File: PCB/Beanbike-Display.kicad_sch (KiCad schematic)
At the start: 5 parts, among them J1 Conn_01x21_Socket, J2 Conn_01x21_Socket, J3 Conn_01x18_Socket, J4 Conn_01x03_Socket, J5 Conn_01x08_Socket

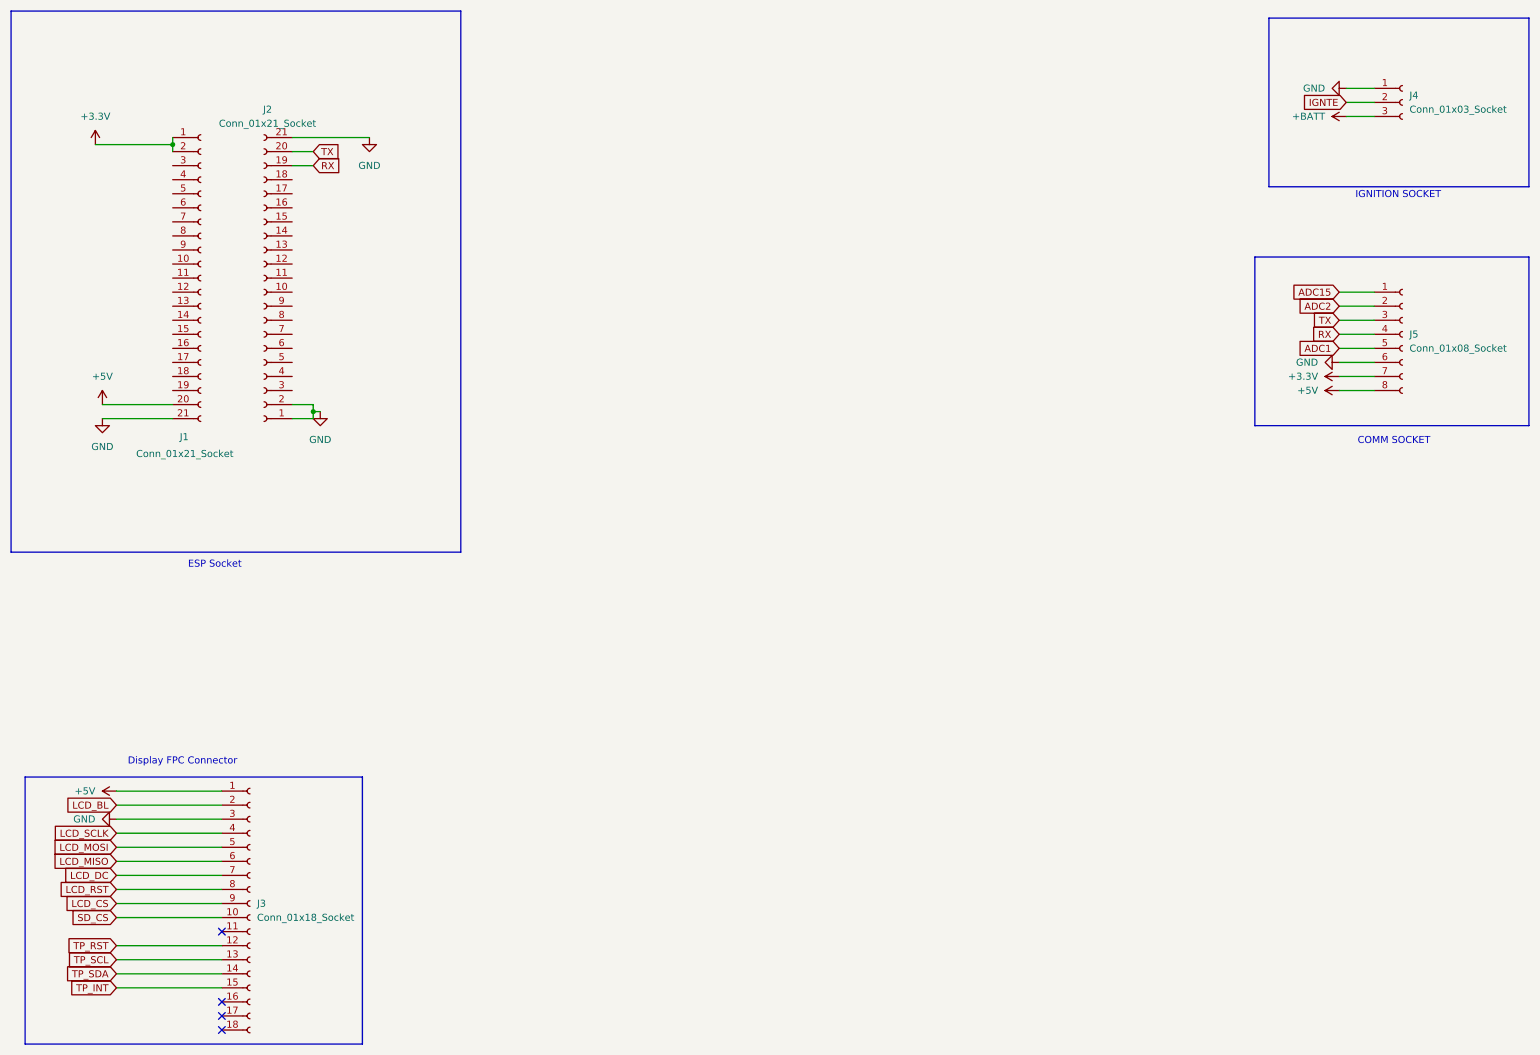
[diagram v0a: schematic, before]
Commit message: PCB v1
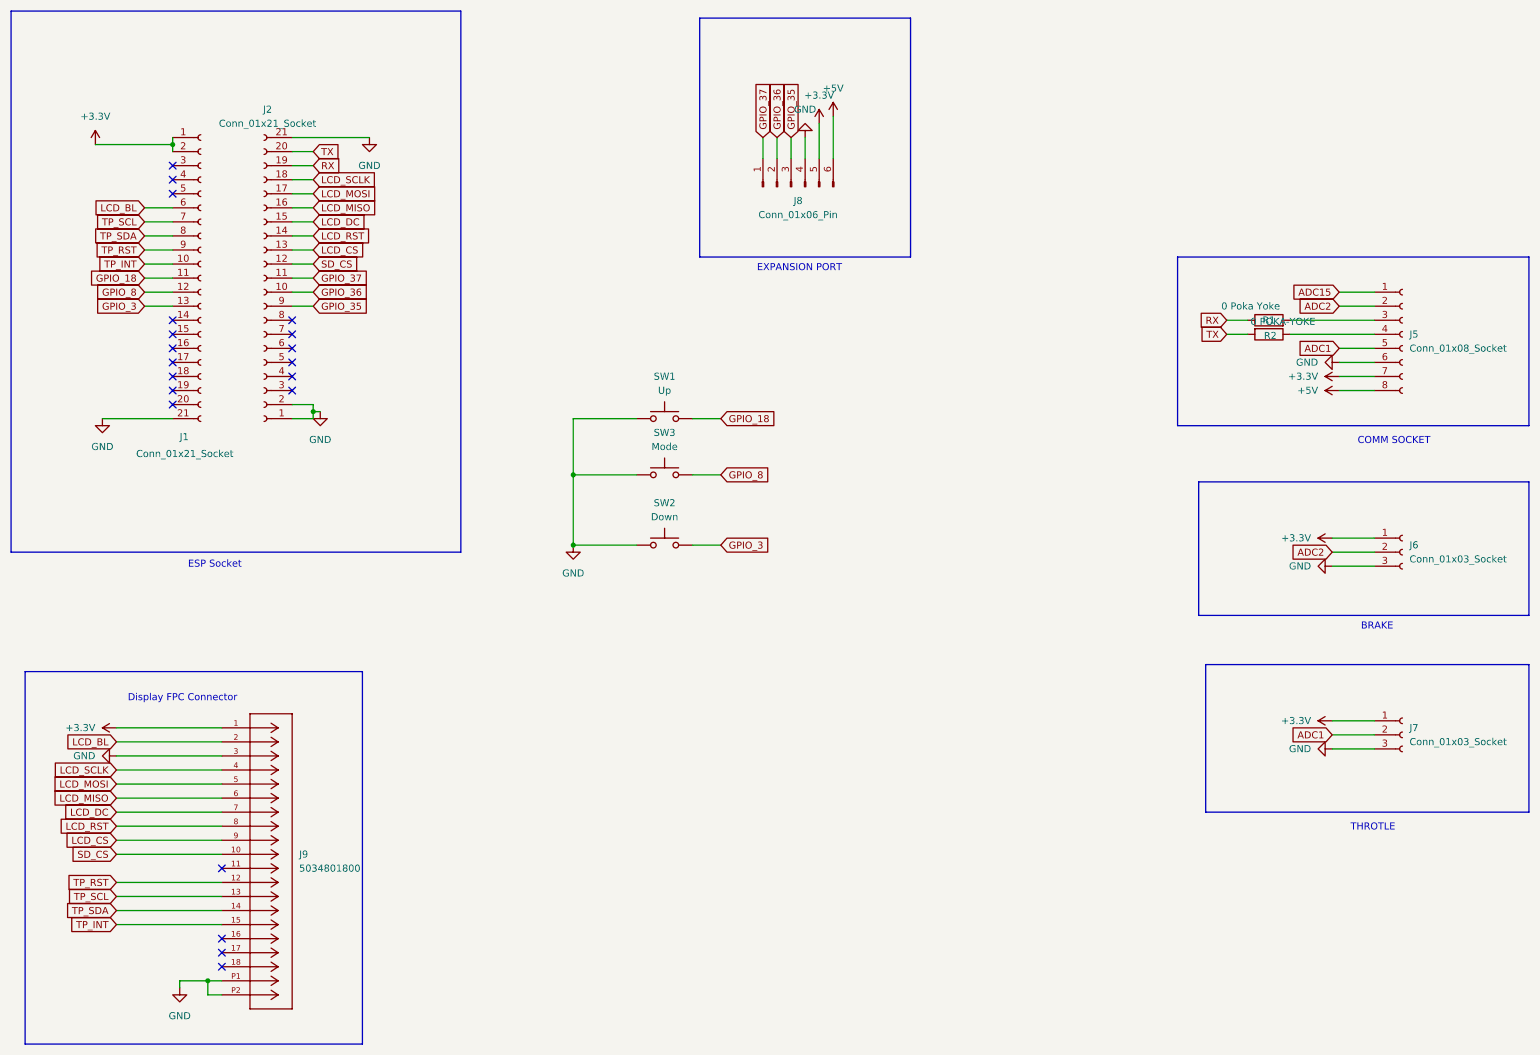
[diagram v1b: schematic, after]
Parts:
- removed J3: Conn_01x18_Socket, symbol Connector:Conn_01x18_Socket
- removed J4: Conn_01x03_Socket, symbol Connector:Conn_01x03_Socket
- added J6, J7: Conn_01x03_Socket, Connector_PinSocket_2.54mm:PinSocket_1x03_P2.54mm_Vertical, symbol Connector:Conn_01x03_Socket
- added J8: Conn_01x06_Pin, Connector_PinHeader_2.54mm:PinHeader_1x06_P2.54mm_Vertical, symbol Connector:Conn_01x06_Pin
- added J9: 5034801800, FPC 0.5mm:CON_5034801800_MOL, symbol FPC_0.5:5034801800
- added R1: 0 Poka Yoke, Resistor_THT:R_Axial_DIN0207_L6.3mm_D2.5mm_P10.16mm_Horizontal, symbol Device:R
- added R2: 0 POKA-YOKE, Resistor_THT:R_Axial_DIN0207_L6.3mm_D2.5mm_P10.16mm_Horizontal, symbol Device:R
- added SW1: Up, Button_Switch_SMD:SW_SPST_PTS645Sx43SMTR92, symbol Switch:SW_Push
- added SW2: Down, Button_Switch_SMD:SW_SPST_PTS645Sx43SMTR92, symbol Switch:SW_Push
- added SW3: Mode, Button_Switch_SMD:SW_SPST_PTS645Sx43SMTR92, symbol Switch:SW_Push
- J1, J2: footprint (none) -> Connector_PinSocket_2.54mm:PinSocket_1x21_P2.54mm_Vertical
- J5: footprint (none) -> Connector_PinSocket_2.54mm:PinSocket_1x08_P2.54mm_Vertical
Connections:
- net +3.3V: now also J6.1 (Pin_1), J7.1 (Pin_1), J8.5 (Pin_5), J9.1
- net +5V: now also J8.6 (Pin_6); no longer J1.20 (Pin_20)
- net ADC1: now also J7.2 (Pin_2)
- net ADC2: now also J6.2 (Pin_2)
- net GND: now also J6.3 (Pin_3), J7.3 (Pin_3), J8.4 (Pin_4), J9.3, J9.P1, J9.P2, SW1.1, SW2.1, SW3.1
- net LCD_BL: now also J1.6 (Pin_6), J9.2
- net LCD_CS: now also J2.13 (Pin_13), J9.9
- net LCD_DC: now also J2.15 (Pin_15), J9.7
- net LCD_MISO: now also J2.16 (Pin_16), J9.6
- net LCD_MOSI: now also J2.17 (Pin_17), J9.5
- net LCD_RST: now also J2.14 (Pin_14), J9.8
- net LCD_SCLK: now also J2.18 (Pin_18), J9.4
- net RX: now also R1.1; no longer J5.4 (Pin_4)
- net SD_CS: now also J2.12 (Pin_12), J9.10
- net TP_INT: now also J1.10 (Pin_10), J9.15
- net TP_RST: now also J1.9 (Pin_9), J9.12
- net TP_SCL: now also J1.7 (Pin_7), J9.13
- net TP_SDA: now also J1.8 (Pin_8), J9.14
- net TX: now also R2.2; no longer J5.3 (Pin_3)
- net GPIO_18: now reaches J1.11 (Pin_11)
- net GPIO_18: now also SW1.2
- net GPIO_8: now reaches J1.12 (Pin_12)
- net GPIO_8: now also SW3.2
- net GPIO_3: now reaches J1.13 (Pin_13)
- net GPIO_3: now also SW2.2
- net GPIO_36: now reaches J2.10 (Pin_10)
- net GPIO_36: now also J8.2 (Pin_2)
- net GPIO_37: now reaches J2.11 (Pin_11)
- net GPIO_37: now also J8.1 (Pin_1)
- net GPIO_35: now reaches J2.9 (Pin_9)
- net GPIO_35: now also J8.3 (Pin_3)
- new net: J5.3 (Pin_3), R1.2
- new net: J5.4 (Pin_4), R2.1
- no-connect marks 4 -> 20
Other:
- note added: "BRAKE"
- note added: "EXPANSION PORT"
- note added: "THROTLE"
- note removed: "IGNITION SOCKET"

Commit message: BikeState & RTOS
I forgot to commit
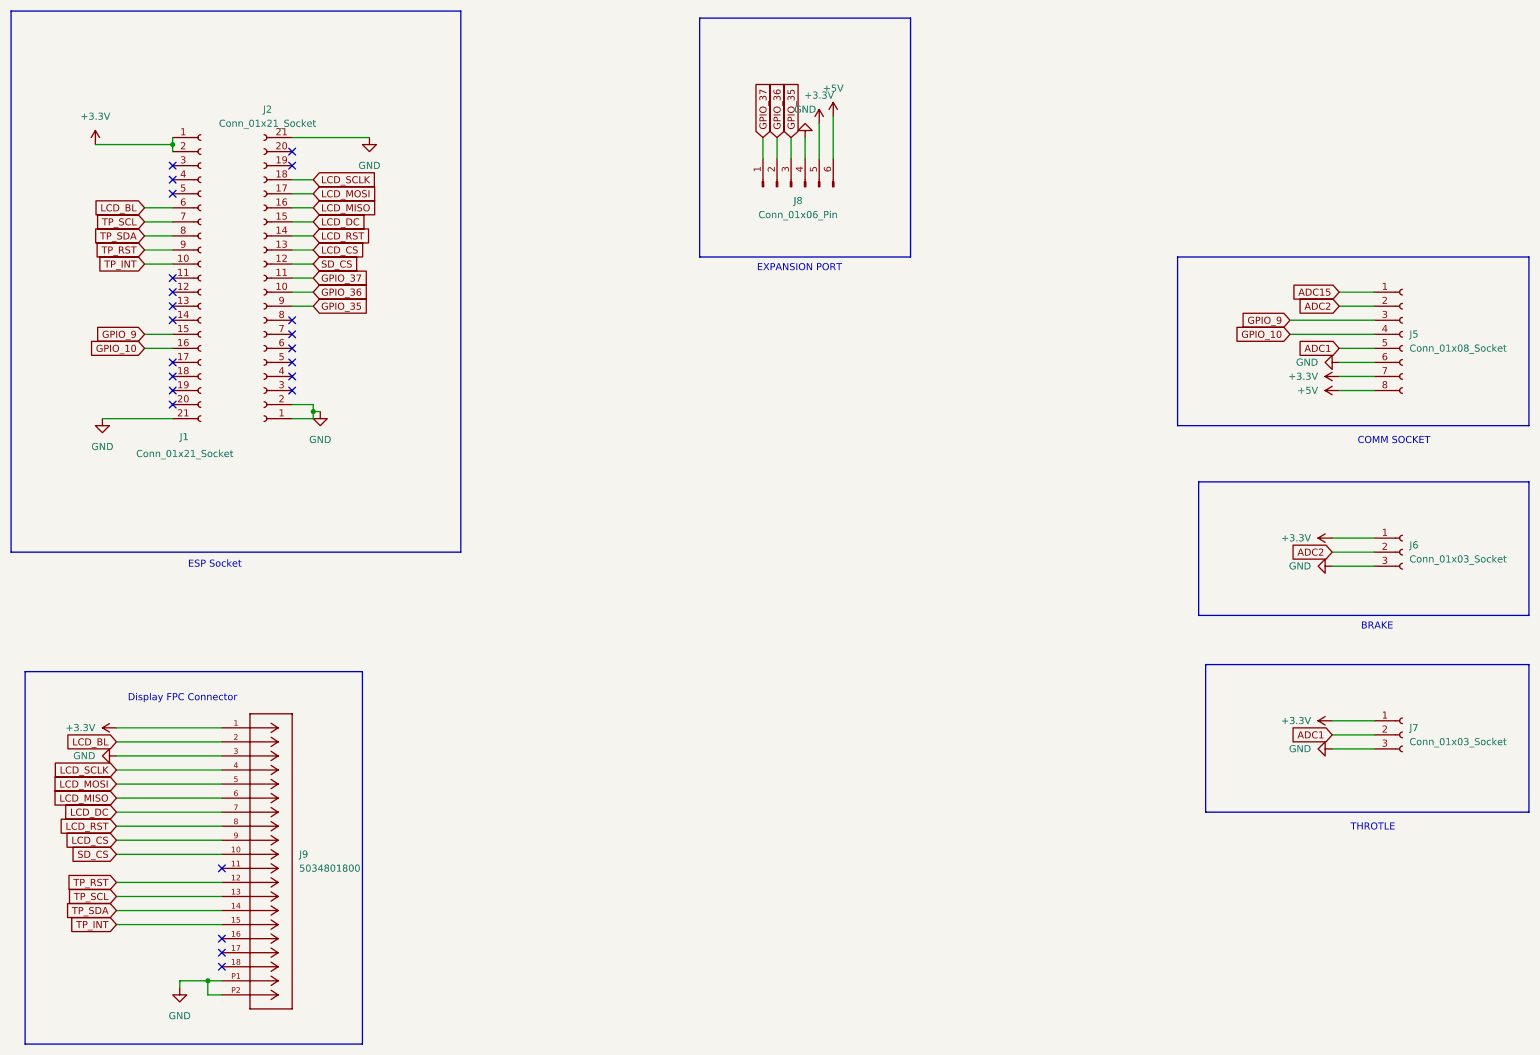
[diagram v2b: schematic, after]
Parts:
- removed R1: 0 Poka Yoke, Resistor_THT:R_Axial_DIN0207_L6.3mm_D2.5mm_P10.16mm_Horizontal, symbol Device:R
- removed R2: 0 POKA-YOKE, Resistor_THT:R_Axial_DIN0207_L6.3mm_D2.5mm_P10.16mm_Horizontal, symbol Device:R
- removed SW1: Up, Button_Switch_SMD:SW_SPST_PTS645Sx43SMTR92, symbol Switch:SW_Push
- removed SW2: Down, Button_Switch_SMD:SW_SPST_PTS645Sx43SMTR92, symbol Switch:SW_Push
- removed SW3: Mode, Button_Switch_SMD:SW_SPST_PTS645Sx43SMTR92, symbol Switch:SW_Push
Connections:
- net GPIO_9: now reaches J5.3 (Pin_3)
- net GPIO_9: now also J1.15 (Pin_15)
- net GPIO_10: now reaches J5.4 (Pin_4)
- net GPIO_10: now also J1.16 (Pin_16)
- net GPIO_18: no longer names the net of J1.11 (Pin_11)
- net GPIO_3: no longer names the net of J1.13 (Pin_13)
- net GPIO_8: no longer names the net of J1.12 (Pin_12)
- net RX: no longer names the net of J2.19 (Pin_19)
- net TX: no longer names the net of J2.20 (Pin_20)
- no-connect marks 20 -> 23
